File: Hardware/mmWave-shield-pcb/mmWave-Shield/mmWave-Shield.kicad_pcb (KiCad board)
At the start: 4 copper layers, 21 x 15 mm, 42 parts, among them J3 DF40HC_3.0_-40DS-0.4V_51, J4 DF40HC_3.0_-50DS-0.4V_51, U1 TPS22916CYFPR, U2 TPS22916CYFPR, X1 KC2016K80.0000C1GE00

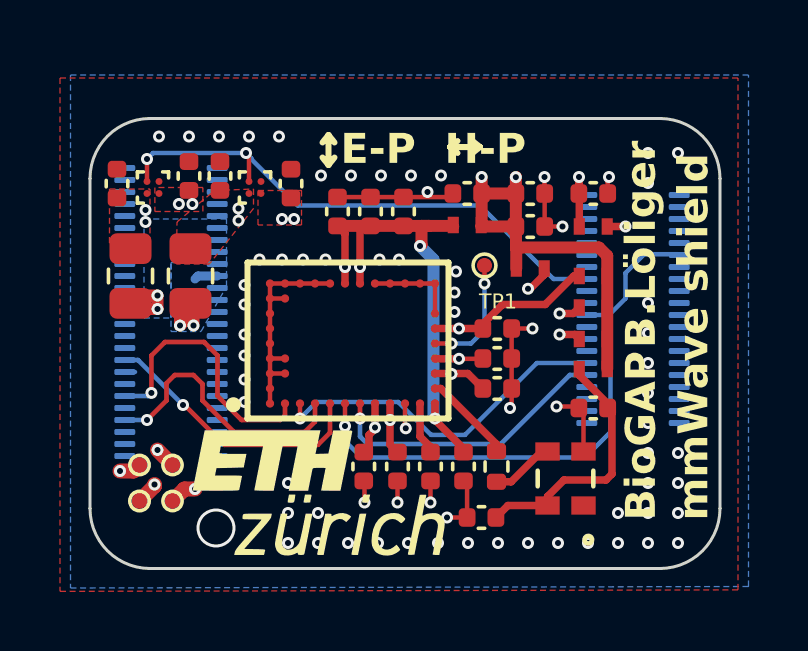
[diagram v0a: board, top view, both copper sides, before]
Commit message: Cleaning up a bit
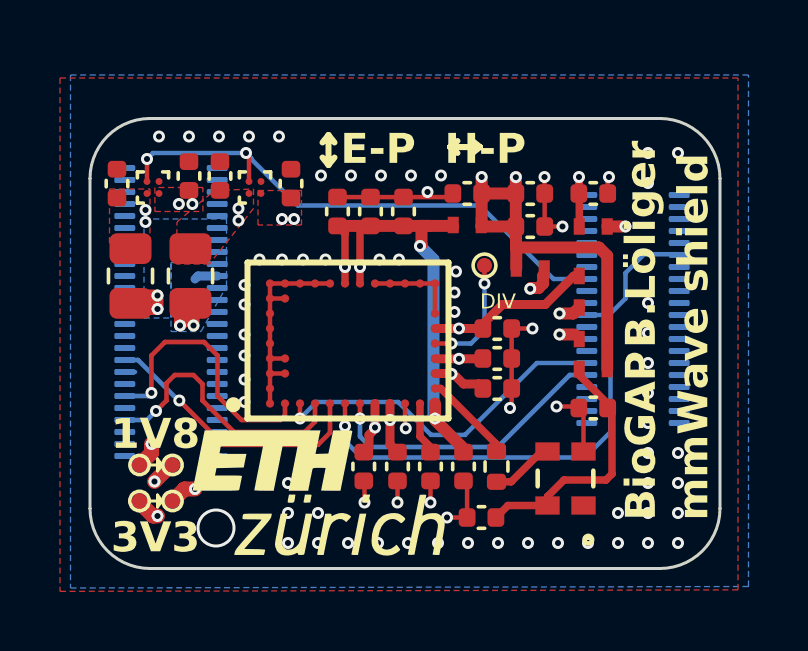
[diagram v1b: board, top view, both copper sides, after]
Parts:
- moved TP4 1.10 mm to (138.6, 105.2)
- moved TP5 1.10 mm to (139.7, 105.2)
- renumbered TP1 to DIV
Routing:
- net /sensor/sw_in_1v8: track 10.2 -> 11.4 mm
- net VD2: track 10.8 -> 11.8 mm
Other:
- board text added: "1V8"
- board text added: "3V3"
